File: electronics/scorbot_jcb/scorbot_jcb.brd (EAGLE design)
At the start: 100 x 80 mm, 12 parts

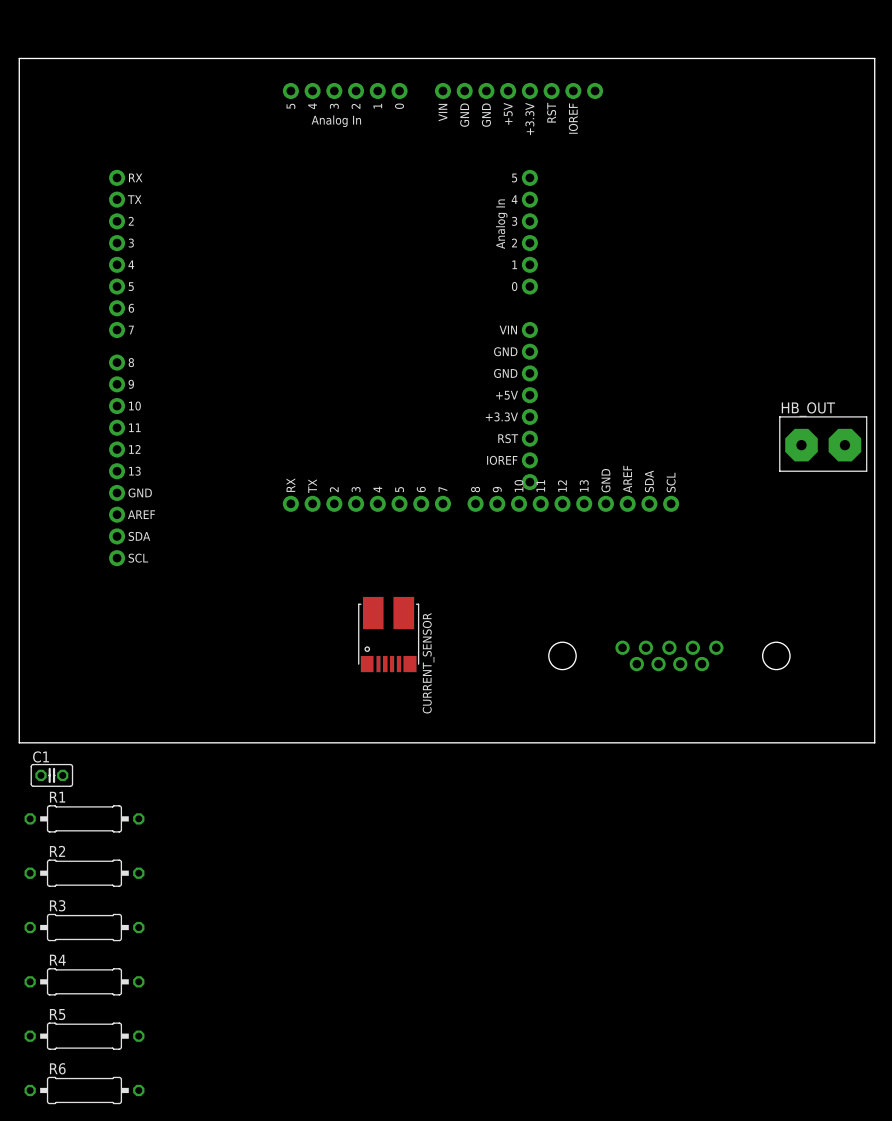
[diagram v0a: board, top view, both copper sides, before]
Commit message: Board init design
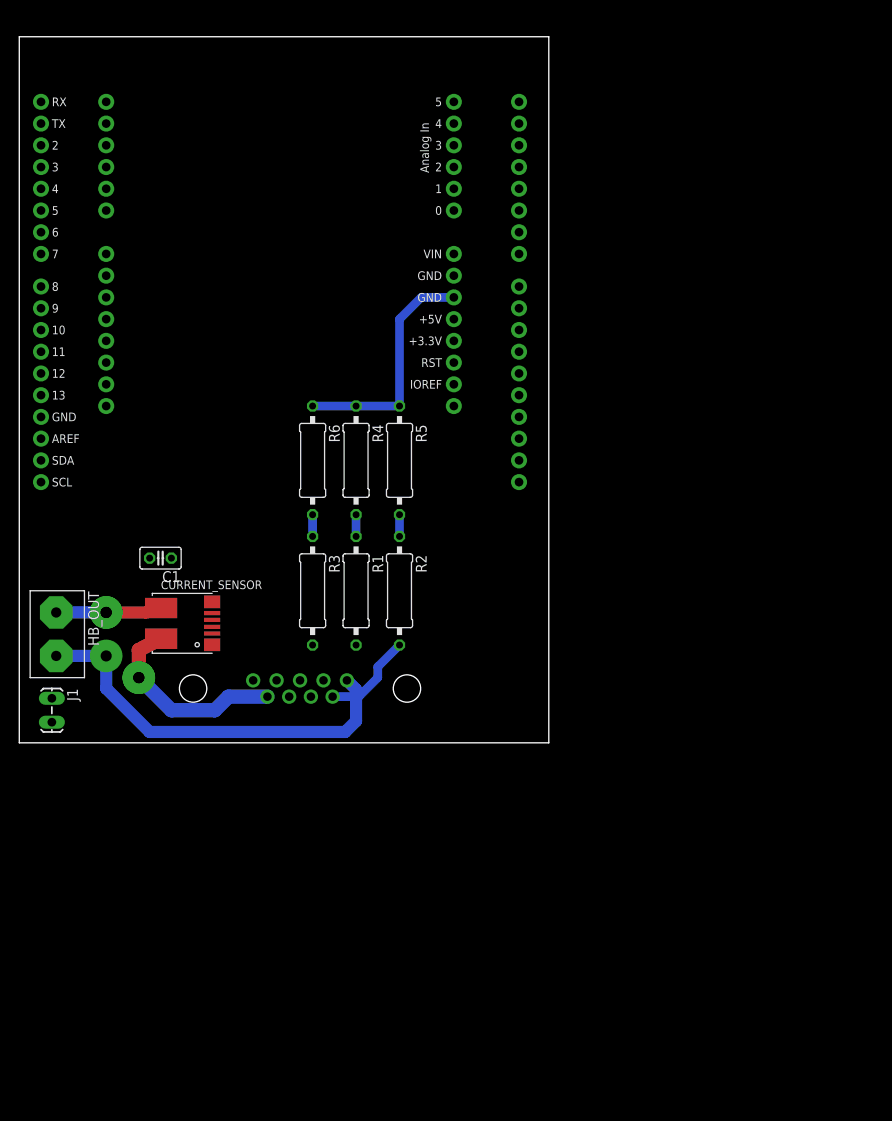
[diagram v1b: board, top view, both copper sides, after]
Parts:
- added J1: (no value), uchile_robotics_eagle_lib:1X02_LOCK_LONGPADS
- moved HB_OUT 93.7 mm to (2.54, 12.7), turned to 270 degrees
- moved XMC4800 86.5 mm to (0.00, 20.3), turned to 0 degrees
- moved R6 78.3 mm to (34.3, 33.0), turned to 270 degrees
- moved R5 76.7 mm to (44.5, 33.0), turned to 270 degrees
- moved R4 68.7 mm to (39.4, 33.0), turned to 270 degrees
- moved HBRIDGE 52.8 mm to (61.0, 20.3), flipped to the bottom
- moved R2 49.5 mm to (44.5, 17.8), turned to 270 degrees
- moved R3 47.6 mm to (34.3, 17.8), turned to 270 degrees
- moved DB9 43.3 mm to (20.3, 6.35)
- moved R1 41.5 mm to (39.4, 17.8), turned to 270 degrees
- moved C1 28.4 mm to (16.5, 21.6), turned to 180 degrees
- moved CURRENT_SENSOR 24.2 mm to (19.1, 14.0), turned to 90 degrees
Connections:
- net +5V: now also J1.1
- net GND: now also J1.2
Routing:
- net N$3: track 0.00 -> 46.7 mm
- net GND: track 0.00 -> 27.7 mm
- net N$1: track 0.00 -> 23.4 mm, vias 0 -> 1
- net N$2: track 0.00 -> 12.3 mm, vias 0 -> 1
- net N$10: track 0.00 -> 11.1 mm
- net HOME: track 0.00 -> 2.54 mm
- net ENC_B: track 0.00 -> 2.54 mm
- net ENC_A: track 0.00 -> 2.54 mm
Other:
- board size 100 x 80 mm -> 61.9 x 82.5 mm

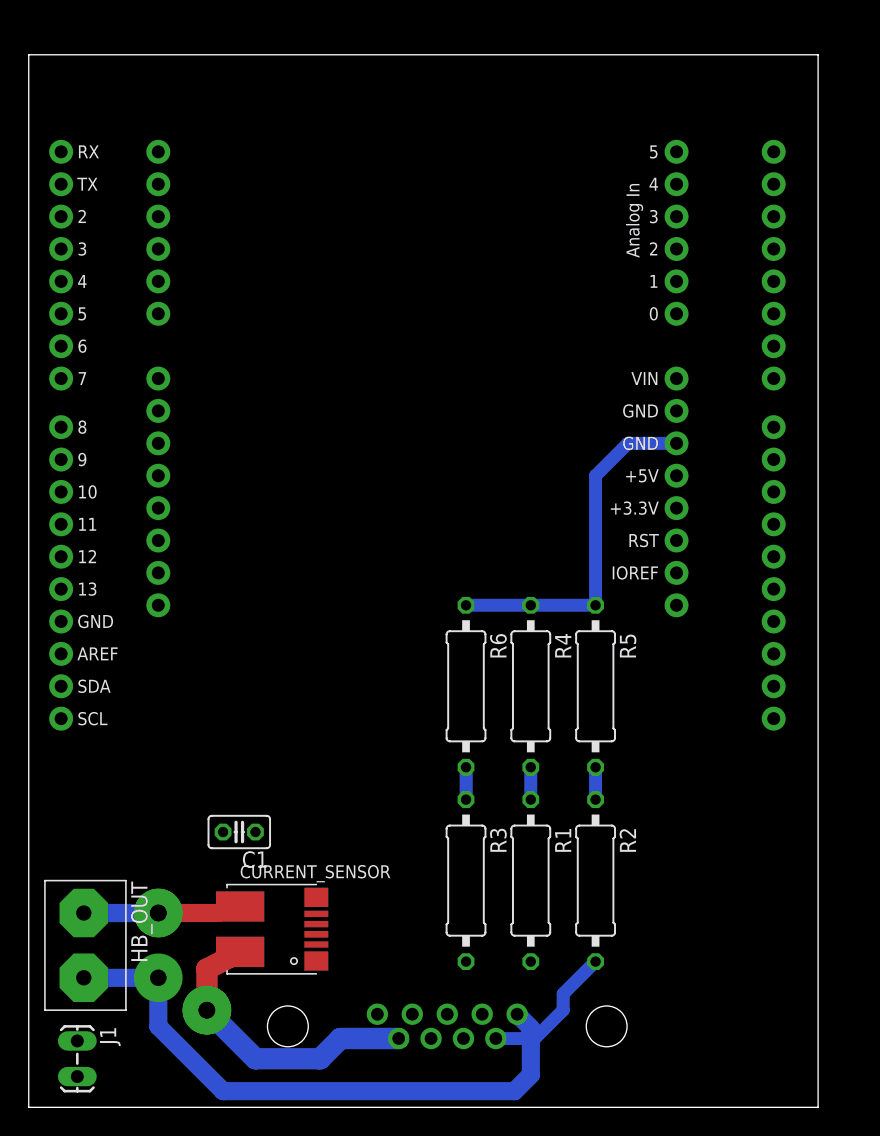
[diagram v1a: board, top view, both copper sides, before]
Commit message: Ruteo
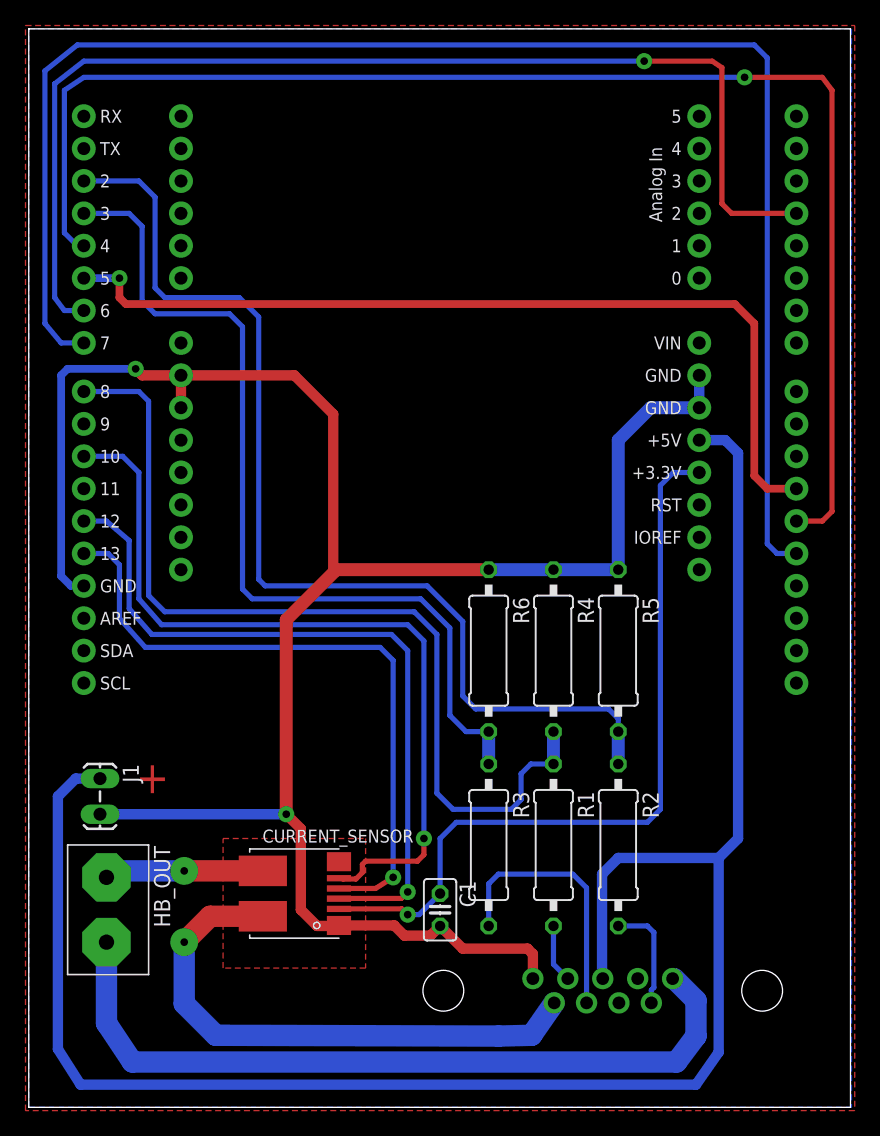
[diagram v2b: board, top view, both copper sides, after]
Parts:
- moved J1 20.7 mm to (5.59, 25.7)
- moved C1 16.9 mm to (32.3, 15.5), turned to 270 degrees
- moved DB9 12.5 mm to (32.5, 9.14)
- moved R1 3.31 mm to (41.1, 20.6)
- moved R4 3.31 mm to (41.1, 35.8)
- moved HBRIDGE 3.31 mm to (62.7, 23.1)
- moved HB_OUT 3.31 mm to (4.32, 15.5)
- moved R2 3.31 mm to (46.2, 20.6)
- moved R3 3.31 mm to (36.1, 20.6)
- moved XMC4800 3.31 mm to (1.78, 23.1)
- moved CURRENT_SENSOR 3.31 mm to (20.8, 16.8)
- moved R5 3.31 mm to (46.2, 35.8)
- moved R6 3.31 mm to (36.1, 35.8)
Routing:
- net +5V: track 0.00 -> 147.3 mm
- net GND: track 27.7 -> 164.0 mm, vias 0 -> 2
- net INH2: track 0.00 -> 122.1 mm
- net INH1: track 0.00 -> 110.3 mm, vias 0 -> 1
- net IN1: track 0.00 -> 89.5 mm, vias 0 -> 1
- net ENC_A: track 2.54 -> 82.6 mm
- net IN2: track 0.00 -> 70.6 mm, vias 0 -> 1
- net HOME: track 2.54 -> 71.8 mm
- net ENC_B: track 2.54 -> 70.6 mm
- net !CS: track 0.00 -> 63.2 mm, vias 0 -> 1
- net +3V3: track 0.00 -> 60.2 mm, vias 0 -> 1
- net MISO: track 0.00 -> 57.3 mm, vias 0 -> 1
- net SCLK: track 0.00 -> 51.8 mm, vias 0 -> 1
- net N$11: track 0.00 -> 20.8 mm
- net N$1: track 23.4 -> 43.2 mm
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- added copper zone on layer 1, net GND
- added copper zone on layer 16, net GND
- added copper zone on layer 1, net N$5
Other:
- board size 61.9 x 82.5 mm -> 64.4 x 84.6 mm
- board text added: "+"
